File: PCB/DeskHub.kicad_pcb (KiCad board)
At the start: 4 copper layers, 212.6 x 108.9 mm, 120 parts, among them J1 USB_A, J2 5V Barrel, J4 USB_A, J5 USB_A, J6 USB_A, J7 USB_A, U1 TUSB4041I, U2 3.3V Reg, U3 1.1V Reg, U4 TPS2001CDGNR, U5 TPS2001CDGNR, U6 TPS2001CDGNR, U7 TPS2001CDGNR, Y1 ECS-240-20-30B-TR

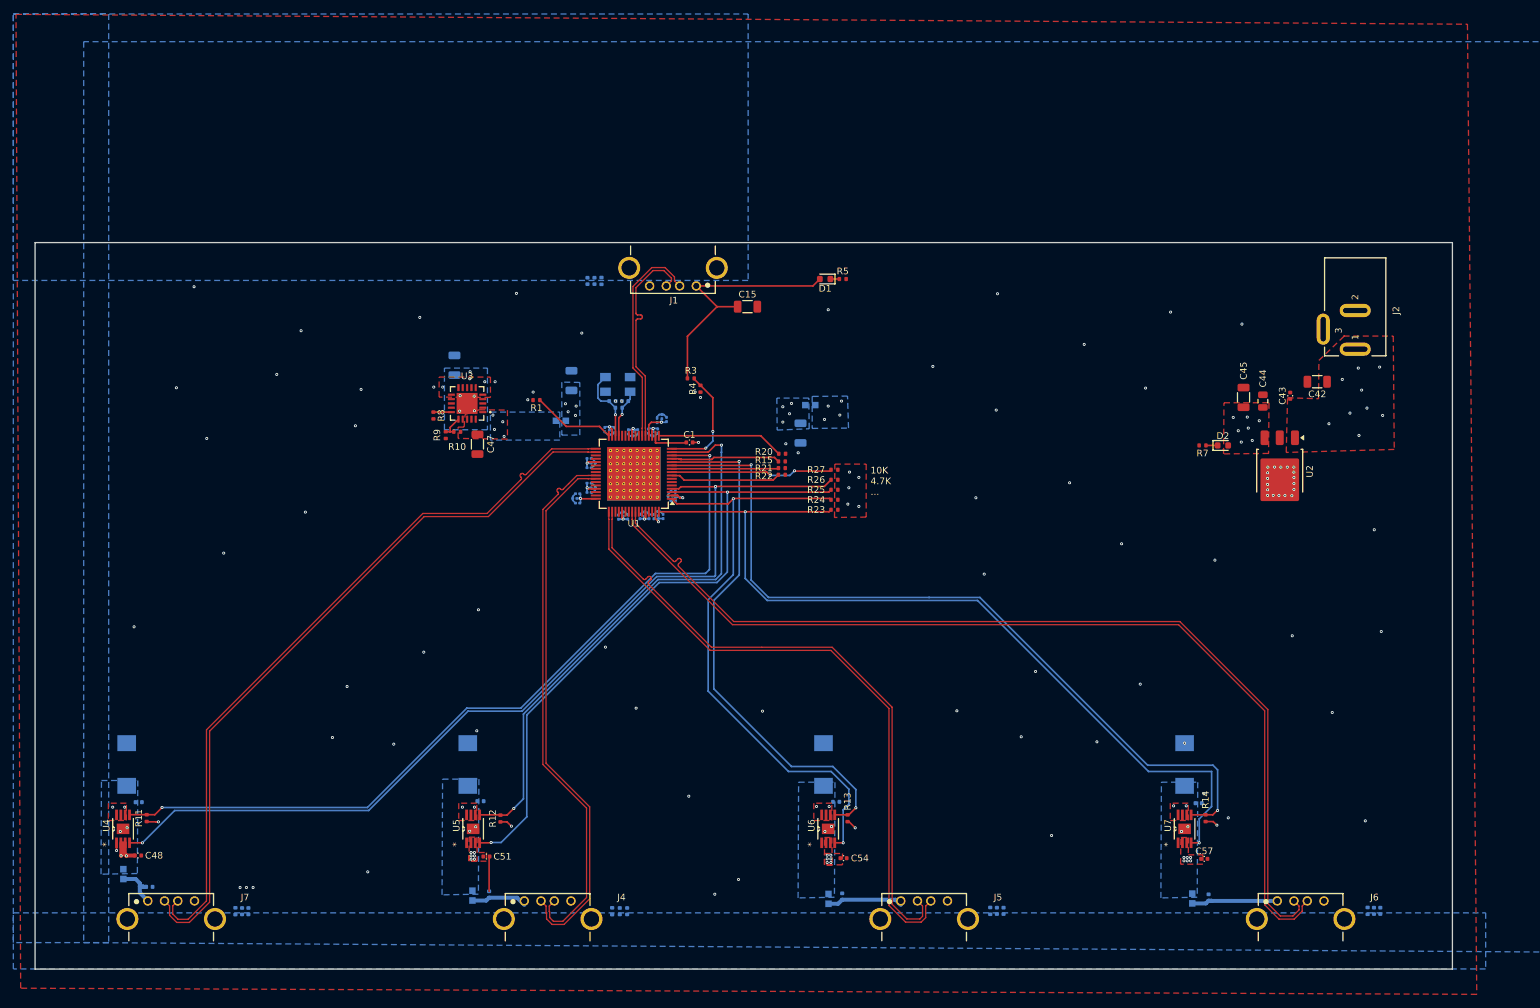
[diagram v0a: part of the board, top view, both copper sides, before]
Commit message: pcb v2.0 condensed
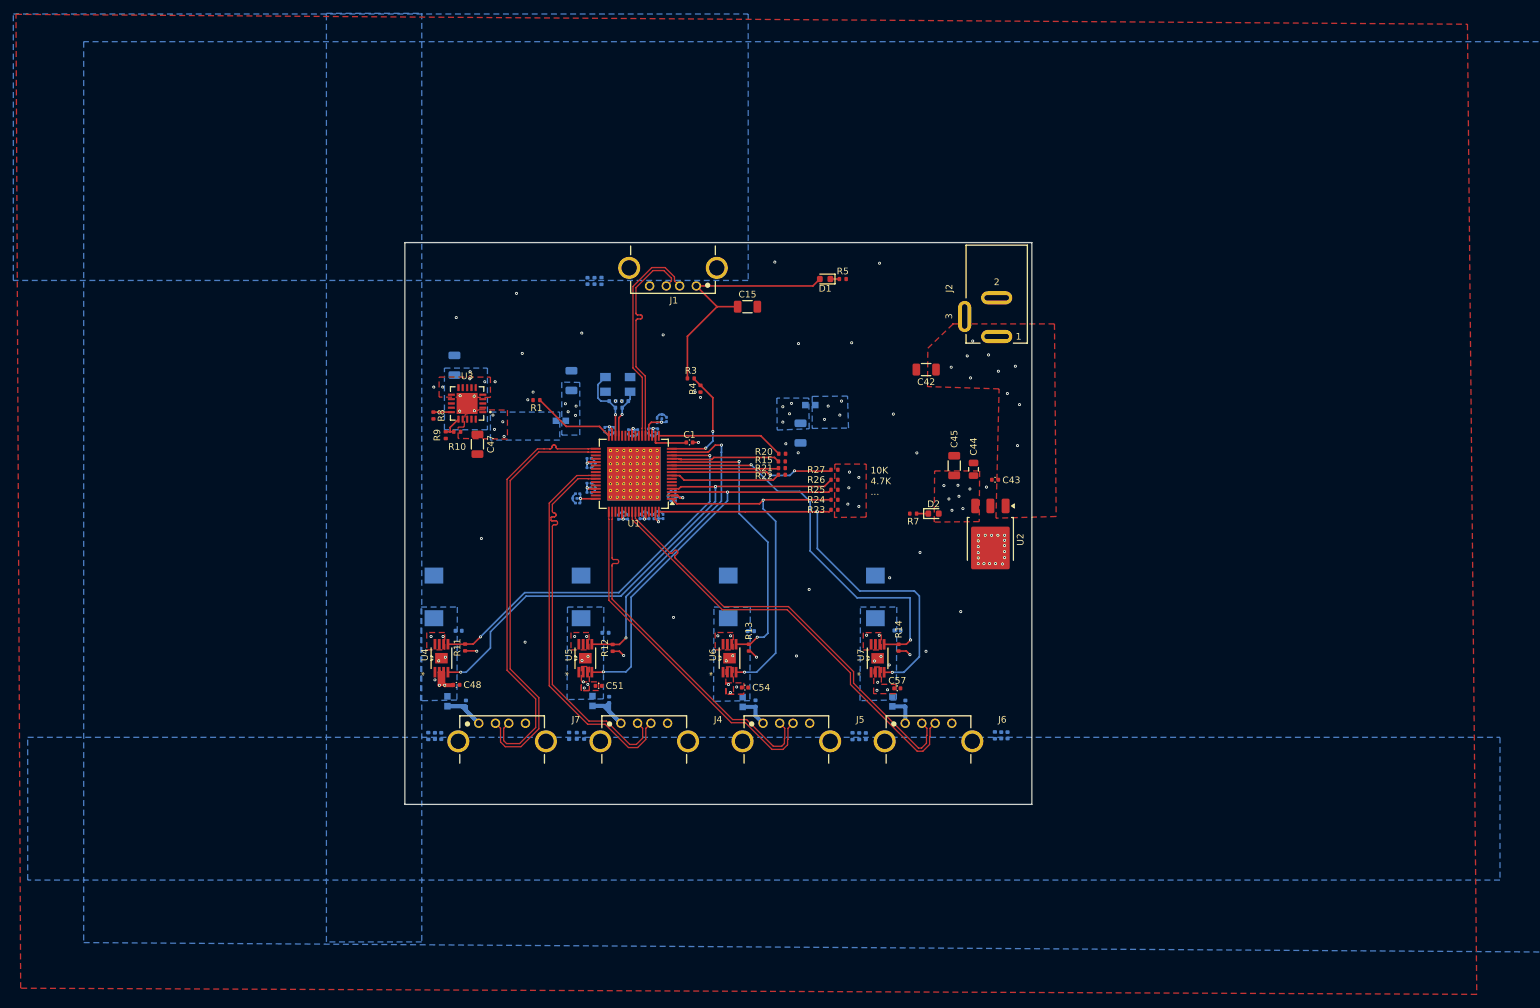
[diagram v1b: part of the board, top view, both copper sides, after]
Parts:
- moved J6 61.8 mm to (187.5, 137.0)
- moved C69 61.8 mm to (199.3, 132.8)
- moved C70 61.8 mm to (198.4, 132.8)
- moved R18 61.8 mm to (197.4, 132.8)
- moved C42 58.7 mm to (187.1, 78.0)
- moved J7 56.3 mm to (123.5, 137.0)
- moved FB7 55.1 mm to (115.3, 127.7)
- moved C74 54.9 mm to (118.1, 128.1), turned to 90 degrees
- moved C49 54.4 mm to (117.0, 117.2)
- moved R11 54.2 mm to (118.0, 119.6)
- moved C48 54.2 mm to (116.7, 125.3)
- moved U4 54.2 mm to (114.5, 121.3)
- moved C71 54.0 mm to (184.0, 128.1)
- moved FB4 53.8 mm to (182.1, 127.8)
- moved J2 53.8 mm to (197.7, 67.2)
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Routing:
- net USB_DN4_D+: track 146.3 -> 65.1 mm
- net USB_DN4_D-: track 146.2 -> 65.1 mm
- net /Port 4 Power Switch/PWRON_EN: track 130.6 -> 65.2 mm
- net /Port 1 Power Switch/OVERCURRENT: track 125.0 -> 60.8 mm
- net /Port 1 Power Switch/PWRON_EN: track 142.3 -> 78.8 mm
- net /Port 4 Power Switch/OVERCURRENT: track 121.4 -> 59.0 mm
- net USB_DN1_D-: track 111.1 -> 63.9 mm
- net USB_DN1_D+: track 111.1 -> 63.9 mm
- net USB_DN3_D-: track 96.7 -> 53.2 mm
- net USB_DN3_D+: track 96.7 -> 53.2 mm
- net /Port 2 Power Switch/OVERCURRENT: track 85.9 -> 48.3 mm
- net /Port 3 Power Switch/PWRON_EN: track 91.9 -> 55.3 mm
- net /Port 3 Power Switch/OVERCURRENT: track 79.7 -> 43.2 mm
- net /Port 2 Power Switch/PWRON_EN: track 98.9 -> 62.4 mm
- net USB_DN2_D-: track 81.8 -> 57.6 mm
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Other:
- board size 212.6 x 108.9 mm -> 94 x 84.2 mm
